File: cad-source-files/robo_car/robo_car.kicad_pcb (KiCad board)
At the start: 2 copper layers, 100 x 100 mm, 94 parts, among them J1 Conn_01x06_MountingPin, J16 Conn_01x02_MountingPin, J2 ftdi_conn, J3 Conn_01x06_MountingPin, J4 Barrel_Jack, J5 Conn_01x04, J6 Conn_01x06_MountingPin, J7 Conn_01x02_MountingPin, J8 Conn_01x02_MountingPin, SW1 SW_Push, SW2 SW_Push, U1 XL1509, U2 AMS1117-3.3, U3 ESP32-WROOM-32U, U4 MOTOR_DRIVER-LV8548MC-AH

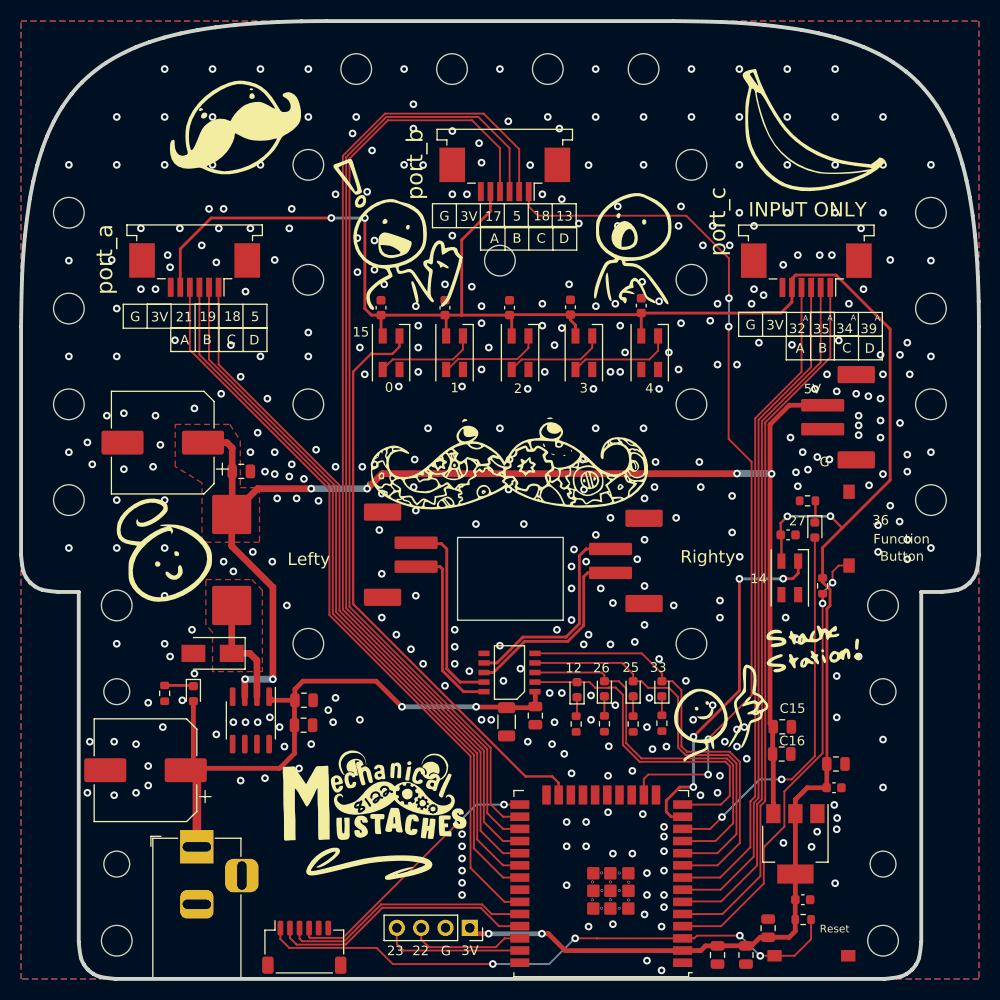
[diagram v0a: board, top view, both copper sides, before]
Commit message: 3rd try lets go
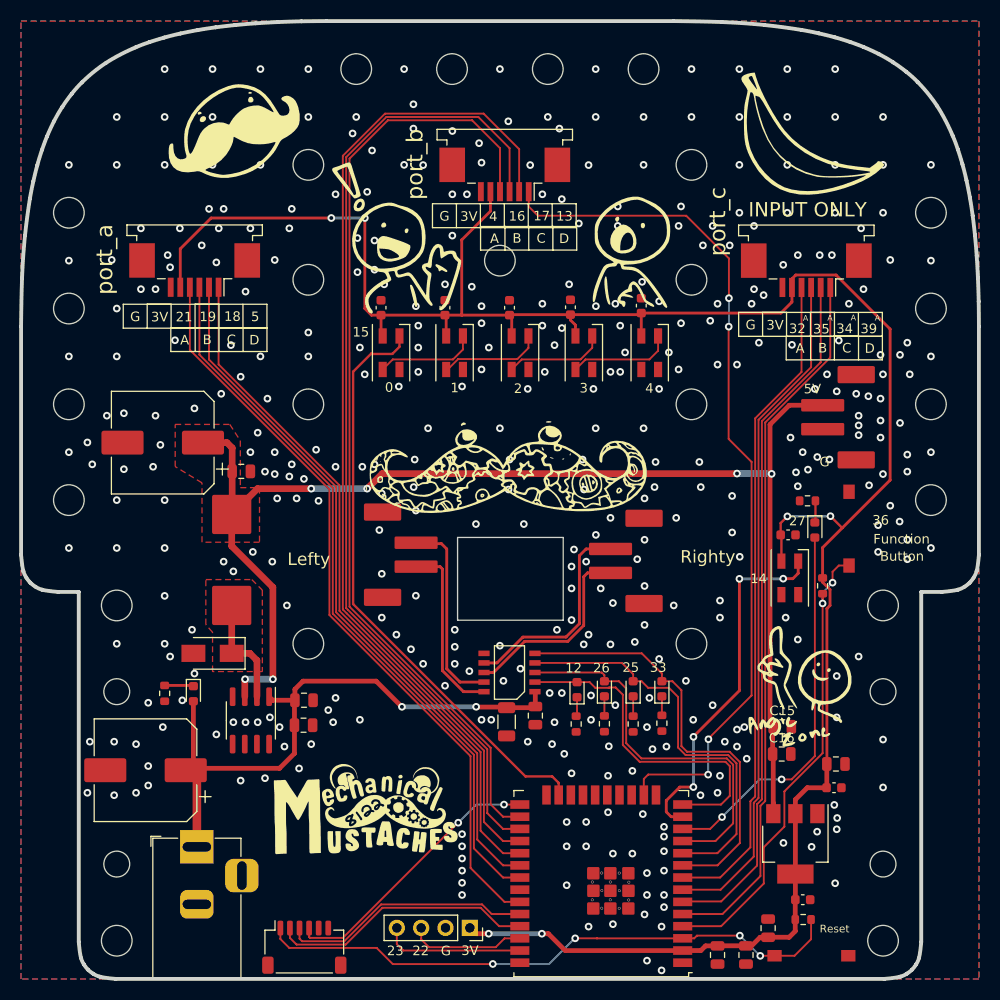
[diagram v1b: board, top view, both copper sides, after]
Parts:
- removed the G*** at (150.3, 98.4)
- removed the G*** at (150.6, 104.0)
- removed the G*** at (150.9, 100.9)
- removed the G*** at (152.4, 102.3)
- added G***: LOGO, Drawing:mustache, F.Cu at (150.8, 101.3)
- moved G*** 1.69 mm to (135.9, 132.9)
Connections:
- net /INPUT_A renamed /IO16
- net /INPUT_B renamed /IO17
- net /INPUT_C renamed /IO4
- net /INPUT_D renamed /IO13
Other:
- board text added: "16"
